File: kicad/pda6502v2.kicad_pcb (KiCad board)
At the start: 2 copper layers, 4 parts, among them U1 W65C02SxP, U2 AS6C62256-55PCN, U3 W65C22SxP, U4 AS6C62256-55PCN

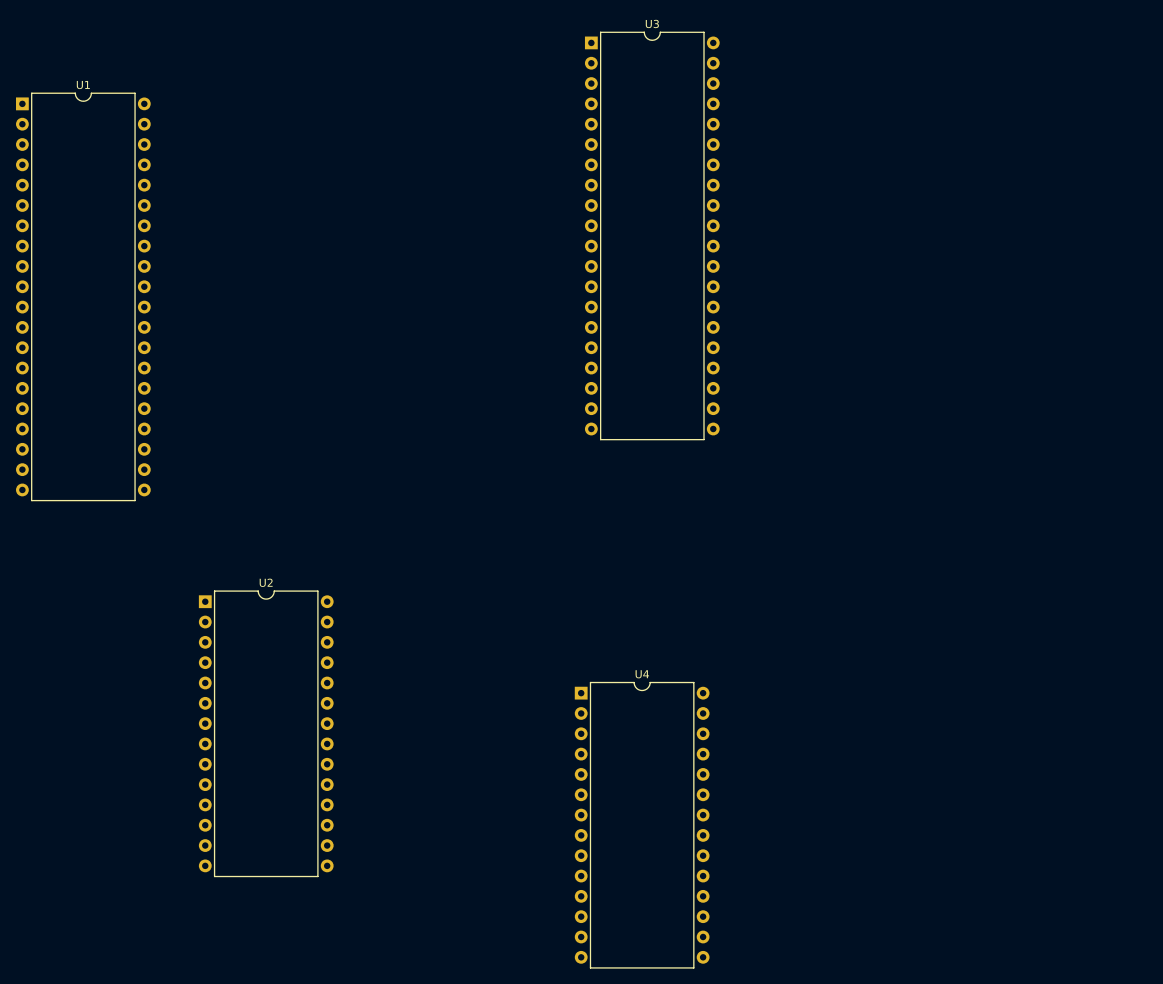
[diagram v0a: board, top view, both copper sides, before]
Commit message: Lots of progress on schematic, some PCB part placement.
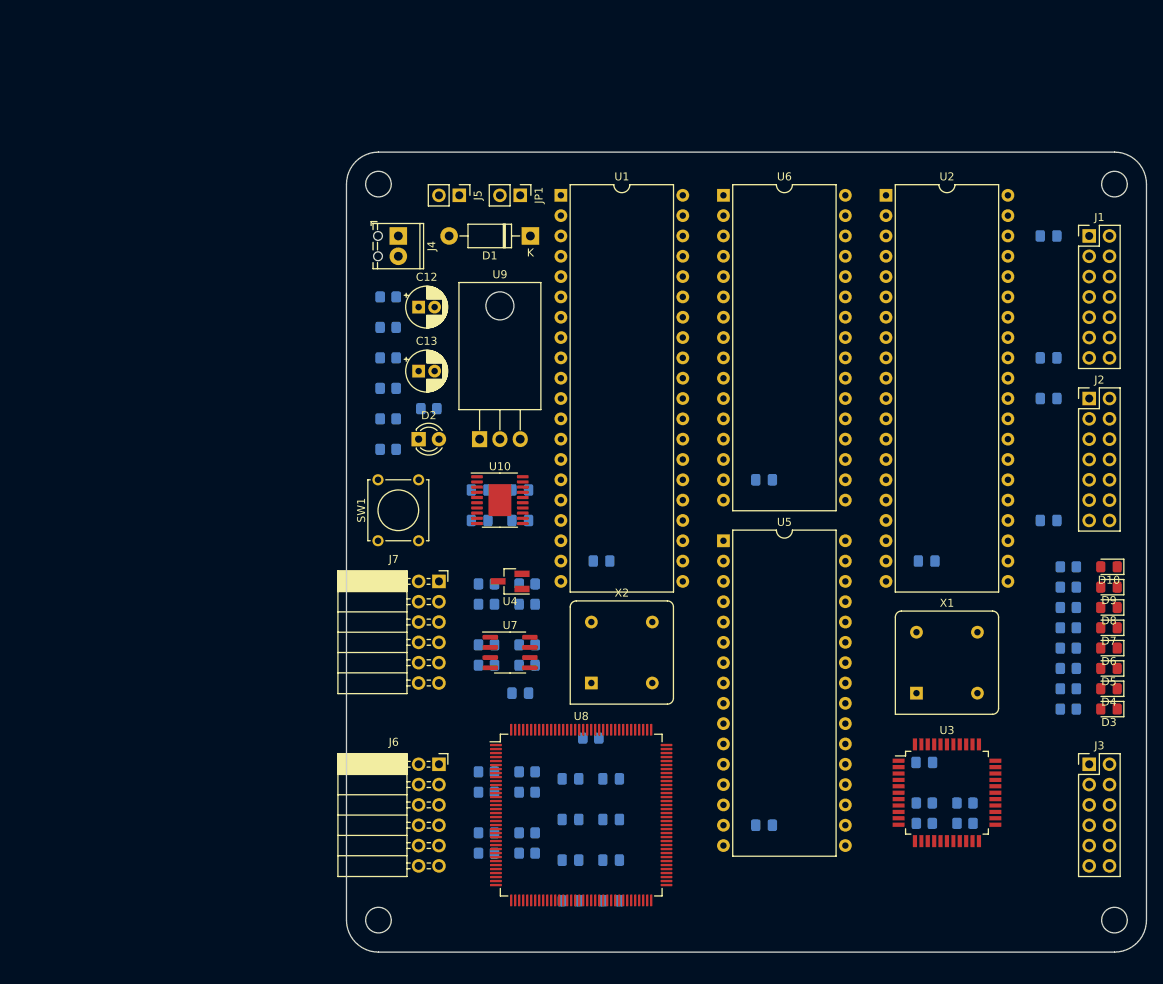
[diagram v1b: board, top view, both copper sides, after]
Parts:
- added C1: 0.1μF, Capacitor_SMD:C_0805_2012Metric_Pad1.18x1.45mm_HandSolder, B.Cu at (129.5, 91.4)
- added C10: 0.1μF, Capacitor_SMD:C_0805_2012Metric_Pad1.18x1.45mm_HandSolder, B.Cu at (119.4, 108.0)
- added C11: 0.1μF, Capacitor_SMD:C_0805_2012Metric_Pad1.18x1.45mm_HandSolder, B.Cu at (125.7, 133.9)
- added C12: 100uF, Capacitor_THT:CP_Radial_D5.0mm_P2.00mm, F.Cu at (106.7, 59.7)
- added C13: 10uF, Capacitor_THT:CP_Radial_D5.0mm_P2.00mm, F.Cu at (106.7, 67.7)
- added C14: 0.1μF, Capacitor_SMD:C_0805_2012Metric_Pad1.18x1.45mm_HandSolder, B.Cu at (125.7, 128.8)
- added C15: 0.1μF, Capacitor_SMD:C_0805_2012Metric_Pad1.18x1.45mm_HandSolder, B.Cu at (125.7, 123.7)
- added C16: 0.1μF, Capacitor_SMD:C_0805_2012Metric_Pad1.18x1.45mm_HandSolder, B.Cu at (125.7, 118.7)
- added C17: 0.1μF, Capacitor_SMD:C_0805_2012Metric_Pad1.18x1.45mm_HandSolder, B.Cu at (130.7, 133.9)
- added C18: 10nF, Capacitor_SMD:C_0805_2012Metric_Pad1.18x1.45mm_HandSolder, B.Cu at (119.4, 86.4)
- added C19: 10nF, Capacitor_SMD:C_0805_2012Metric_Pad1.18x1.45mm_HandSolder, B.Cu at (119.4, 82.5)
- added C2: 0.1μF, Capacitor_SMD:C_0805_2012Metric_Pad1.18x1.45mm_HandSolder, B.Cu at (170.2, 91.4)
- added C20: 10uF, Capacitor_SMD:C_0805_2012Metric_Pad1.18x1.45mm_HandSolder, B.Cu at (114.3, 86.4)
- added C21: 10uF, Capacitor_SMD:C_0805_2012Metric_Pad1.18x1.45mm_HandSolder, B.Cu at (114.3, 82.5)
- added C22: 0.1μF, Capacitor_SMD:C_0805_2012Metric_Pad1.18x1.45mm_HandSolder, B.Cu at (130.7, 128.8)
- added C23: 0.1μF, Capacitor_SMD:C_0805_2012Metric_Pad1.18x1.45mm_HandSolder, B.Cu at (130.7, 123.7)
- added C24: 0.1μF, Capacitor_SMD:C_0805_2012Metric_Pad1.18x1.45mm_HandSolder, B.Cu at (130.7, 118.7)
- added C3: 0.1μF, Capacitor_SMD:C_0805_2012Metric_Pad1.18x1.45mm_HandSolder, B.Cu at (169.9, 116.6)
- added C4: 0.1μF, Capacitor_SMD:C_0805_2012Metric_Pad1.18x1.45mm_HandSolder, B.Cu at (149.9, 124.5)
- added C5: 0.1μF, Capacitor_SMD:C_0805_2012Metric_Pad1.18x1.45mm_HandSolder, B.Cu at (185.4, 50.8)
- added C6: 0.1μF, Capacitor_SMD:C_0805_2012Metric_Pad1.18x1.45mm_HandSolder, B.Cu at (185.4, 71.1)
- added C7: 0.1μF, Capacitor_SMD:C_0805_2012Metric_Pad1.18x1.45mm_HandSolder, B.Cu at (185.4, 66.0)
- added C8: 0.1μF, Capacitor_SMD:C_0805_2012Metric_Pad1.18x1.45mm_HandSolder, B.Cu at (185.4, 86.4)
- added C9: 0.1μF, Capacitor_SMD:C_0805_2012Metric_Pad1.18x1.45mm_HandSolder, B.Cu at (149.9, 81.3)
- added D1: 1N5819, Diode_THT:D_DO-41_SOD81_P10.16mm_Horizontal, F.Cu at (120.7, 50.8)
- added D10: LED, LED_SMD:LED_0805_2012Metric_Pad1.15x1.40mm_HandSolder, F.Cu at (193.0, 92.2)
- added D2: LED, LED_THT:LED_D3.0mm, F.Cu at (106.7, 76.2)
- added D3: LED, LED_SMD:LED_0805_2012Metric_Pad1.15x1.40mm_HandSolder, F.Cu at (193.0, 109.9)
- added D4: LED, LED_SMD:LED_0805_2012Metric_Pad1.15x1.40mm_HandSolder, F.Cu at (193.0, 107.4)
- added D5: LED, LED_SMD:LED_0805_2012Metric_Pad1.15x1.40mm_HandSolder, F.Cu at (193.0, 104.9)
- added D6: LED, LED_SMD:LED_0805_2012Metric_Pad1.15x1.40mm_HandSolder, F.Cu at (193.0, 102.3)
- added D7: LED, LED_SMD:LED_0805_2012Metric_Pad1.15x1.40mm_HandSolder, F.Cu at (193.0, 99.8)
- added D8: LED, LED_SMD:LED_0805_2012Metric_Pad1.15x1.40mm_HandSolder, F.Cu at (193.0, 97.2)
- added D9: LED, LED_SMD:LED_0805_2012Metric_Pad1.15x1.40mm_HandSolder, F.Cu at (193.0, 94.7)
- added J1: GPIOA, Connector_PinHeader_2.54mm:PinHeader_2x07_P2.54mm_Vertical, F.Cu at (190.5, 50.8)
- added J2: GPIOB, Connector_PinHeader_2.54mm:PinHeader_2x07_P2.54mm_Vertical, F.Cu at (190.5, 71.1)
- added J3: UART, Connector_PinHeader_2.54mm:PinHeader_2x06_P2.54mm_Vertical, F.Cu at (190.5, 116.8)
- added J4: Screw_Terminal_01x02, TerminalBlock_Phoenix:TerminalBlock_Phoenix_MPT-0,5-2-2.54_1x02_P2.54mm_Horizontal, F.Cu at (104.1, 50.8)
- added J5: Conn_01x02, Connector_PinHeader_2.54mm:PinHeader_1x02_P2.54mm_Vertical, F.Cu at (111.8, 45.7)
- added J6: PMOD A, Connector_PinSocket_2.54mm:PinSocket_2x06_P2.54mm_Horizontal, F.Cu at (109.2, 116.8)
- added J7: PMOD B, Connector_PinSocket_2.54mm:PinSocket_2x06_P2.54mm_Horizontal, F.Cu at (109.2, 94.0)
- added JP1: Jumper, Connector_PinHeader_2.54mm:PinHeader_1x02_P2.54mm_Vertical, F.Cu at (119.4, 45.7)
- added R1: 10K, Resistor_SMD:R_0805_2012Metric_Pad1.20x1.40mm_HandSolder, B.Cu at (169.9, 121.7)
- added R10: 100Ω, Resistor_SMD:R_0805_2012Metric_Pad1.20x1.40mm_HandSolder, B.Cu at (115.2, 94.3)
- added R11: 100Ω, Resistor_SMD:R_0805_2012Metric_Pad1.20x1.40mm_HandSolder, B.Cu at (120.2, 96.8)
- added R12: 100Ω, Resistor_SMD:R_0805_2012Metric_Pad1.20x1.40mm_HandSolder, B.Cu at (115.2, 96.8)
- added R13: 100Ω, Resistor_SMD:R_0805_2012Metric_Pad1.20x1.40mm_HandSolder, B.Cu at (120.2, 120.3)
- added R14: 100Ω, Resistor_SMD:R_0805_2012Metric_Pad1.20x1.40mm_HandSolder, B.Cu at (115.2, 120.3)
- added R15: 100Ω, Resistor_SMD:R_0805_2012Metric_Pad1.20x1.40mm_HandSolder, B.Cu at (120.2, 117.8)
- added R16: 100Ω, Resistor_SMD:R_0805_2012Metric_Pad1.20x1.40mm_HandSolder, B.Cu at (115.2, 117.8)
- added R17: 100Ω, Resistor_SMD:R_0805_2012Metric_Pad1.20x1.40mm_HandSolder, B.Cu at (120.2, 101.9)
- added R18: 100Ω, Resistor_SMD:R_0805_2012Metric_Pad1.20x1.40mm_HandSolder, B.Cu at (115.2, 101.9)
- added R19: 100Ω, Resistor_SMD:R_0805_2012Metric_Pad1.20x1.40mm_HandSolder, B.Cu at (120.2, 104.5)
- added R2: 10K, Resistor_SMD:R_0805_2012Metric_Pad1.20x1.40mm_HandSolder, B.Cu at (175.0, 121.7)
- added R20: 100Ω, Resistor_SMD:R_0805_2012Metric_Pad1.20x1.40mm_HandSolder, B.Cu at (115.2, 104.5)
- added R21: 10K, Resistor_SMD:R_0805_2012Metric_Pad1.20x1.40mm_HandSolder, B.Cu at (102.9, 58.4)
- added R22: 10K, Resistor_SMD:R_0805_2012Metric_Pad1.20x1.40mm_HandSolder, B.Cu at (102.9, 62.2)
- added R23: 10K, Resistor_SMD:R_0805_2012Metric_Pad1.20x1.40mm_HandSolder, B.Cu at (128.2, 113.6)
- added R24: ?, Resistor_SMD:R_0805_2012Metric_Pad1.20x1.40mm_HandSolder, B.Cu at (102.9, 66.0)
- added R25: ?, Resistor_SMD:R_0805_2012Metric_Pad1.20x1.40mm_HandSolder, B.Cu at (102.9, 69.8)
- added R26: ?, Resistor_SMD:R_0805_2012Metric_Pad1.20x1.40mm_HandSolder, B.Cu at (102.9, 73.7)
- added R27: ?, Resistor_SMD:R_0805_2012Metric_Pad1.20x1.40mm_HandSolder, B.Cu at (102.9, 77.5)
- added R28: 1K, Resistor_SMD:R_0805_2012Metric_Pad1.20x1.40mm_HandSolder, B.Cu at (108.0, 72.4)
- added R29: 1K, Resistor_SMD:R_0805_2012Metric_Pad1.20x1.40mm_HandSolder, B.Cu at (187.9, 109.9)
- added R3: 10K, Resistor_SMD:R_0805_2012Metric_Pad1.20x1.40mm_HandSolder, B.Cu at (169.9, 124.2)
- added R30: 1K, Resistor_SMD:R_0805_2012Metric_Pad1.20x1.40mm_HandSolder, B.Cu at (187.9, 107.4)
- added R31: 1K, Resistor_SMD:R_0805_2012Metric_Pad1.20x1.40mm_HandSolder, B.Cu at (187.9, 104.9)
- added R32: 1K, Resistor_SMD:R_0805_2012Metric_Pad1.20x1.40mm_HandSolder, B.Cu at (187.9, 102.3)
- added R33: 1K, Resistor_SMD:R_0805_2012Metric_Pad1.20x1.40mm_HandSolder, B.Cu at (187.9, 99.8)
- added R34: 1K, Resistor_SMD:R_0805_2012Metric_Pad1.20x1.40mm_HandSolder, B.Cu at (187.9, 97.2)
- added R35: 1K, Resistor_SMD:R_0805_2012Metric_Pad1.20x1.40mm_HandSolder, B.Cu at (187.9, 94.7)
- added R36: 1K, Resistor_SMD:R_0805_2012Metric_Pad1.20x1.40mm_HandSolder, B.Cu at (187.9, 92.2)
- added R4: 10K, Resistor_SMD:R_0805_2012Metric_Pad1.20x1.40mm_HandSolder, B.Cu at (175.0, 124.2)
- added R5: 100Ω, Resistor_SMD:R_0805_2012Metric_Pad1.20x1.40mm_HandSolder, B.Cu at (120.2, 128.0)
- added R6: 100Ω, Resistor_SMD:R_0805_2012Metric_Pad1.20x1.40mm_HandSolder, B.Cu at (115.2, 128.0)
- added R7: 100Ω, Resistor_SMD:R_0805_2012Metric_Pad1.20x1.40mm_HandSolder, B.Cu at (120.2, 125.4)
- added R8: 100Ω, Resistor_SMD:R_0805_2012Metric_Pad1.20x1.40mm_HandSolder, B.Cu at (115.2, 125.4)
- added R9: 100Ω, Resistor_SMD:R_0805_2012Metric_Pad1.20x1.40mm_HandSolder, B.Cu at (120.2, 94.3)
- added REF**: MountingHole_3.2mm_M3, MountingHole:MountingHole_3.2mm_M3, F.Cu at (193.7, 136.3)
- added REF**: MountingHole_3.2mm_M3, MountingHole:MountingHole_3.2mm_M3, F.Cu at (101.7, 136.3)
- added REF**: MountingHole_3.2mm_M3, MountingHole:MountingHole_3.2mm_M3, F.Cu at (193.7, 44.3)
- added REF**: MountingHole_3.2mm_M3, MountingHole:MountingHole_3.2mm_M3, F.Cu at (101.7, 44.3)
- added SW1: SW_Push, Button_Switch_THT:SW_Tactile_Straight_KSA0Axx1LFTR, F.Cu at (101.6, 88.9)
- added U10: LT3030, Package_SO:HTSSOP-20-1EP_4.4x6.5mm_P0.65mm_EP2.85x4mm, F.Cu at (116.8, 83.8)
- added U5: AS6C4002-55PCN, Package_DIP:DIP-32_W15.24mm, F.Cu at (144.8, 88.9)
- added U6: AS6C4008-55PCN, Package_DIP:DIP-32_W15.24mm, F.Cu at (144.8, 45.7)
- added U7: AT25M01, Package_SO:SOIC-8_3.9x4.9mm_P1.27mm, F.Cu at (118.1, 102.9)
- added U8: ICE40HX4K-TQ144, Package_QFP:TQFP-144_20x20mm_P0.5mm, F.Cu at (127.0, 123.2)
- added U9: LM1117-3.3, Package_TO_SOT_THT:TO-220-3_Horizontal_TabDown, F.Cu at (114.3, 76.2)
- added X1: 3.6864 MHz, Oscillator:Oscillator_DIP-8, F.Cu at (168.9, 108.0)
- added X2: 10 MHz, Oscillator:Oscillator_DIP-8, F.Cu at (128.3, 106.7)
- U2: value AS6C62256-55PCN -> W65C22SxP; footprint Package_DIP:DIP-28_W15.24mm -> Package_DIP:DIP-40_W15.24mm
- U3: value W65C22SxP -> SC28L92A1B; footprint Package_DIP:DIP-40_W15.24mm -> Package_QFP:PQFP-44_10x10mm_P0.8mm
- U4: value AS6C62256-55PCN -> DS1818; footprint Package_DIP:DIP-28_W15.24mm -> Package_TO_SOT_SMD:SOT-23_Handsoldering
- moved U3 103.7 mm to (172.7, 120.4)
- moved U2 99.1 mm to (165.1, 45.7)
- moved U1 68.3 mm to (124.5, 45.7)
- moved U4 16.6 mm to (118.1, 94.0), turned to 180 degrees
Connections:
- U1 pad 1: Net-(U1-Pad1) -> /~VECPULL
- U1 pad 10: /ADDR1 -> /A1
- U1 pad 11: /ADDR2 -> /A2
- U1 pad 12: /ADDR3 -> /A3
- U1 pad 13: /ADDR4 -> /A4
- U1 pad 14: /ADDR5 -> /A5
- U1 pad 15: /ADDR6 -> /A6
- U1 pad 16: /ADDR7 -> /A7
- U1 pad 17: /ADDR8 -> /A8
- U1 pad 18: /ADDR9 -> /A9
- U1 pad 19: /ADDR10 -> /A10
- U1 pad 2: Net-(U1-Pad2) -> /READY
- U1 pad 20: /ADDR11 -> /A11
- U1 pad 22: /ADDR12 -> /A12
- U1 pad 23: /ADDR13 -> /A13
- U1 pad 24: /ADDR14 -> /A14
- U1 pad 25: /ADDR15 -> /A15
- U1 pad 26: /DATA7 -> /D7
- U1 pad 27: /DATA6 -> /D6
- U1 pad 28: /DATA5 -> /D5
- U1 pad 29: /DATA4 -> /D4
- U1 pad 30: /DATA3 -> /D3
- U1 pad 31: /DATA2 -> /D2
- U1 pad 32: /DATA1 -> /D1
- U1 pad 33: /DATA0 -> /D0
- U1 pad 34: Net-(U1-Pad34) -> /R~W
- U1 pad 36: Net-(U1-Pad36) -> /BUSEN
- U1 pad 37: /CLK -> /CLOCK
- U1 pad 38: Net-(U1-Pad38) -> /~SETOV
- U1 pad 4: Net-(U1-Pad4) -> /~IRQ
- U1 pad 40: /RESET -> /~RESET
- U1 pad 5: Net-(U1-Pad5) -> /~MLOCK
- U1 pad 6: Net-(U1-Pad6) -> /~NMIRQ
- U1 pad 7: Net-(U1-Pad7) -> /SYNC
- U1 pad 9: /ADDR0 -> /A0
- U2 pad 1: /ADDR14 -> GND
- U2 pad 10: /ADDR0 -> /PORTB_0
- U2 pad 11: /DATA0 -> /PORTB_1
- U2 pad 12: /DATA1 -> /PORTB_2
- U2 pad 13: /DATA2 -> /PORTB_3
- U2 pad 14: GND -> /PORTB_4
- U2 pad 15: /DATA3 -> /PORTB_5
- U2 pad 16: /DATA4 -> /PORTB_6
- U2 pad 17: /DATA5 -> /PORTB_7
- U2 pad 18: /DATA6 -> /PORTB_C1
- U2 pad 19: /DATA7 -> /PORTB_C2
- U2 pad 2: /ADDR12 -> /PORTA_0
- U2 pad 20: /RAM_LO_~CS -> +3V3
- U2 pad 21: /ADDR10 -> /VIA_~IRQ
- U2 pad 22: /RAM_LO_~CS -> /R~W
- U2 pad 23: /ADDR11 -> /VIA_~CS
- U2 pad 24: /ADDR9 -> +3V3
- U2 pad 25: /ADDR8 -> /CLOCK
- U2 pad 26: /ADDR13 -> /D7
- U2 pad 27: /RWB -> /D6
- U2 pad 28: +3V3 -> /D5
- U2 pad 3: /ADDR7 -> /PORTA_1
- U2 pad 4: /ADDR6 -> /PORTA_2
- U2 pad 5: /ADDR5 -> /PORTA_3
- U2 pad 6: /ADDR4 -> /PORTA_4
- U2 pad 7: /ADDR3 -> /PORTA_5
- U2 pad 8: /ADDR2 -> /PORTA_6
- U2 pad 9: /ADDR1 -> /PORTA_7
- U3 pad 1: GND -> /A3
- U3 pad 10: Net-(U3-Pad10) -> /UART_TXB~IRQ
- U3 pad 11: Net-(U3-Pad11) -> /UART_IM
- U3 pad 12: Net-(U3-Pad12) -> /D1
- U3 pad 13: Net-(U3-Pad13) -> /D3
- U3 pad 14: Net-(U3-Pad14) -> /D5
- U3 pad 15: Net-(U3-Pad15) -> /D7
- U3 pad 16: Net-(U3-Pad16) -> GND
- U3 pad 17: Net-(U3-Pad17) -> GND
- U3 pad 18: Net-(U3-Pad18) -> /UART_~IRQ
- U3 pad 19: Net-(U3-Pad19) -> /D6
- U3 pad 2: Net-(U3-Pad2) -> /UARTA_CTS
- U3 pad 20: +3V3 -> /D4
- U3 pad 21: Net-(U3-Pad21) -> /D2
- U3 pad 22: Net-(U3-Pad22) -> /D0
- U3 pad 24: Net-(U3-Pad24) -> /UART_TXA~IRQ
- U3 pad 25: /CLK -> /UART_RXA~IRQ
- U3 pad 26: /DATA7 -> Net-(U3-Pad26)
- U3 pad 27: /DATA6 -> /UARTA_RTS
- U3 pad 28: /DATA5 -> /UARTA_TX
- U3 pad 29: /DATA4 -> /UARTA_RX
- U3 pad 3: Net-(U3-Pad3) -> /UART_~WRN
- U3 pad 30: /DATA3 -> Net-(U3-Pad30)
- U3 pad 31: /DATA2 -> Net-(U3-Pad31)
- U3 pad 32: /DATA1 -> /RESET
- U3 pad 33: /DATA0 -> /UART_~CS
- U3 pad 35: /ADDR3 -> Net-(U3-Pad35)
- U3 pad 36: /ADDR2 -> Net-(U3-Pad36)
- U3 pad 37: /ADDR1 -> Net-(U3-Pad37)
- U3 pad 38: /ADDR0 -> +3V3
- U3 pad 39: Net-(U3-Pad39) -> +3V3
- U3 pad 4: Net-(U3-Pad4) -> /UART_~RDN
- U3 pad 40: Net-(U3-Pad40) -> /A0
- U3 pad 5: Net-(U3-Pad5) -> /UARTB_RX
- U3 pad 6: Net-(U3-Pad6) -> /UARTB_TX
- U3 pad 7: Net-(U3-Pad7) -> /UARTB_RTS
- U3 pad 9: Net-(U3-Pad9) -> /UART_RXB~IRQ
- U4 pad 1: /ADDR14 -> /~RESET
- U4 pad 2: /ADDR12 -> +3V3
- U4 pad 3: /ADDR7 -> GND
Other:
- board outline added: 100 x 100 mm
- copper layers 2 -> 4
- board text added: "pda6502v2"
